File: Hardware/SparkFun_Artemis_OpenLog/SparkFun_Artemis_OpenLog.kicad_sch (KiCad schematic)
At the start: 100 parts, among them J1 CONN_021X02_NO_SILK, J11 QWIIC_CONNECTORJS-1MM, J14 CORTEX_JTAG, J2 JST_2MM_MALE, J3 CONN_021X02_NO_SILK, J4 CONN_06NO_SILK_NO_POP, J5 USB_C_4-LAYER_PADS, J6 MICRO-SD, J7 CONN_01PTH_NO_SILK_YES_STOP, Q1 20V/0.2A/8MHz/1.2Ω/1Vth, Q10 20V/0.2A/8MHz/1.2Ω/1Vth, Q2 20V/4.2A/52mΩ/1.4W, Q3 20V/0.2A/8MHz/1.2Ω/1Vth, Q7 20V/0.2A/8MHz/1.2Ω/1Vth, Q9 20V/0.2A/8MHz/1.2Ω/1Vth, U1 3.0V Supervisor, U10 CH340E, U13 9DoF IMU, U14 1.8V/100mA, U2 MCP73831, U3 3.3V, U4 3.3V, U8 ARTEMIS_MODULE, Y3 32.768kHz

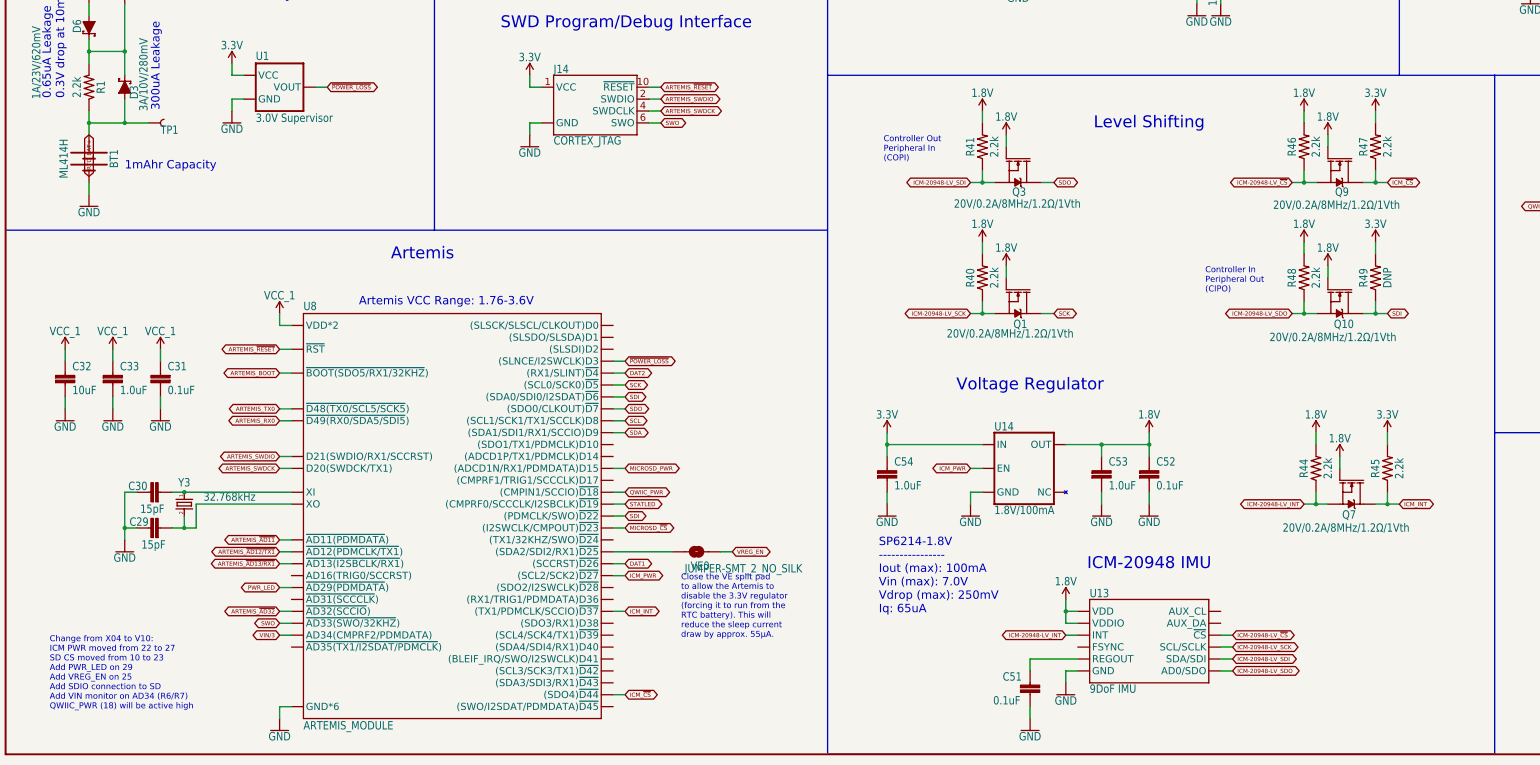
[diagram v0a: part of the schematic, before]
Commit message: Updates the design export
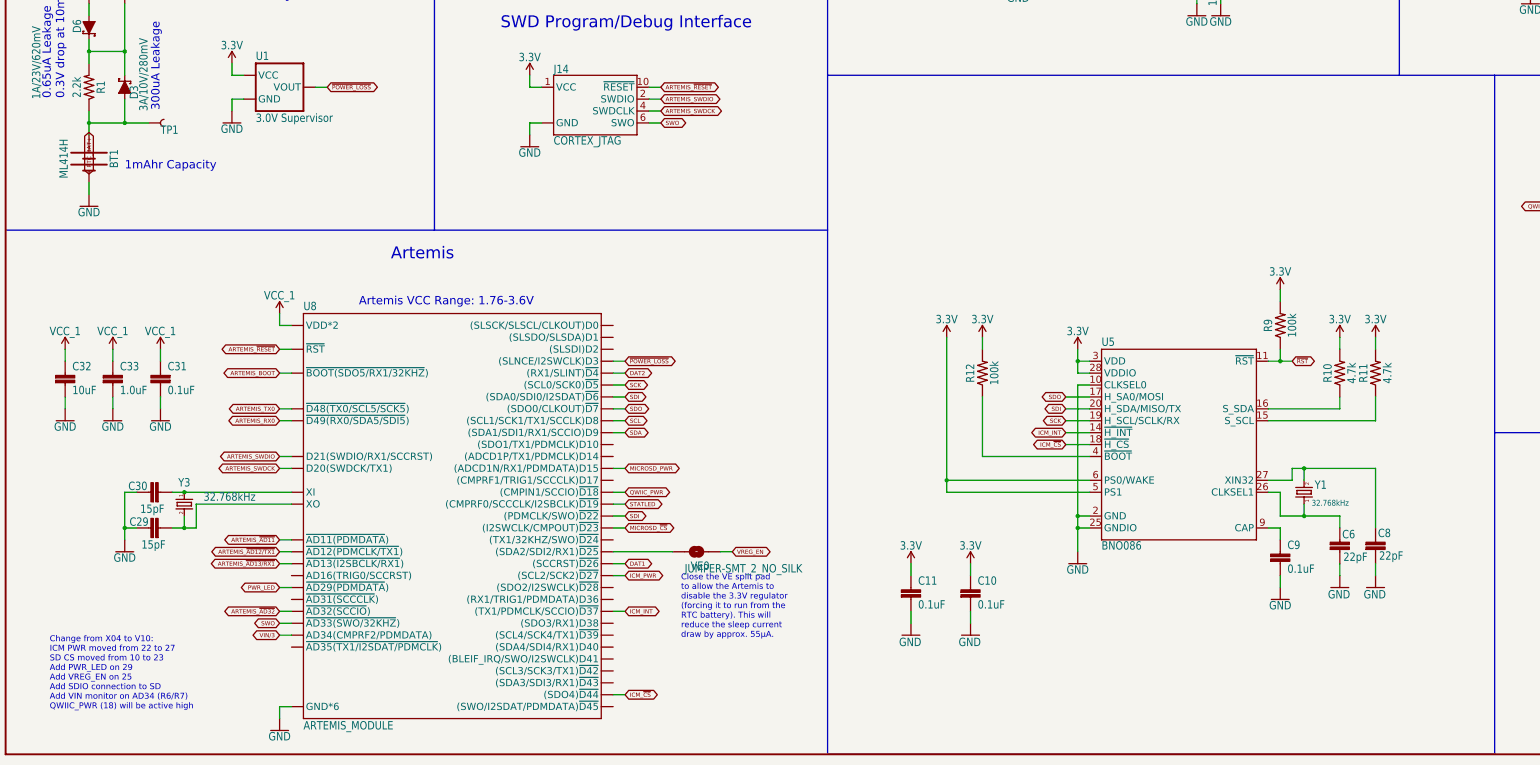
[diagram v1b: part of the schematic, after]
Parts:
- removed C51, C52: 0.1uF, SparkFun_Artemis_OpenLog:0402-TIGHT, symbol SparkFun_Artemis_OpenLog-eagle-import:0.1UF-0402T-16V-10%
- removed C53, C54: 1.0uF, SparkFun_Artemis_OpenLog:0402-TIGHT, symbol SparkFun_Artemis_OpenLog-eagle-import:1.0UF-0402T-16V-10%
- removed Q1, Q10, Q3, Q7, Q9: 20V/0.2A/8MHz/1.2Ω/1Vth, SparkFun_Artemis_OpenLog:SOT-416FL, symbol SparkFun_Artemis_OpenLog-eagle-import:MOSFET-NCH-RE1C00UNTL
- removed R40, R41, R44, R45, R46, R47, R48: 2.2k, SparkFun_Artemis_OpenLog:0402-TIGHT, symbol SparkFun_Artemis_OpenLog-eagle-import:2.2KOHM-0402T-1/16W-1%
- removed R49: DNP, SparkFun_Artemis_OpenLog:0402-TIGHT, symbol SparkFun_Artemis_OpenLog-eagle-import:RESISTOR0402T
- removed U13: 9DoF IMU, SparkFun_Artemis_OpenLog:QFN24-3X3-ICM-20948, symbol SparkFun_Artemis_OpenLog-eagle-import:ICM-20948
- removed U14: 1.8V/100mA, SparkFun_Artemis_OpenLog:SC70, symbol SparkFun_Artemis_OpenLog-eagle-import:V_REG_SP6214-1.8V
- added C10, C11, C9: 0.1uF, SparkFun_Artemis_OpenLog:0402, symbol SparkFun_Artemis_OpenLog-eagle-import:0.1UF-0402-6.3V-10%-X7R
- added C6, C8: 22pF, SparkFun_Artemis_OpenLog:0402-TIGHT, symbol SparkFun_Artemis_OpenLog-eagle-import:22PF-0402T-16V-10%
- added R10, R11: 4.7k, SparkFun_Artemis_OpenLog:0402-TIGHT, symbol SparkFun_Artemis_OpenLog-eagle-import:4.7KOHM-0402T-1/16W-1%
- added R12, R9: 100k, SparkFun_Artemis_OpenLog:0402-TIGHT, symbol SparkFun_Artemis_OpenLog-eagle-import:100KOHM-0402T-1/16W-1%
- added U5: BNO086, SparkFun_Artemis_OpenLog:LGA-28, symbol SparkFun_Artemis_OpenLog-eagle-import:BNO086
- added Y1: 32.768kHz, SparkFun_Artemis_OpenLog:CRYSTAL-SMD-3.2X1.5MM, symbol SparkFun_Artemis_OpenLog-eagle-import:CRYSTAL-32.768KHZSMD-3.2X1.5
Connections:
- net 3.3V: now also C10.1, C11.1, R10.2, R11.2, R12.2, R9.2, U5.28 (VDDIO), U5.3 (VDD), U5.5 (PS1), U5.6 (PS0/WAKE)
- net GND: now also C10.2, C11.2, C6.2, C8.2, C9.2, U5.10 (CLKSEL0), U5.2 (GND), U5.25 (GNDIO)
- net ICM_INT: now also U5.14 (~{H_INT})
- net ICM_~{CS}: now also U5.18 (~{H_CS})
- net SCK: now also U5.19 (H_SCL/SCLK/RX)
- net SDI: now also U5.20 (H_SDA/MISO/TX)
- net SDO: now also U5.17 (H_SA0/MOSI)
- new net: C6.1, U5.26 (CLKSEL1), Y1.P$1 (1)
- new net: C8.1, U5.27 (XIN32), Y1.P$2 (2)
- new net: R11.1, U5.15 (S_SCL)
- new net: R10.1, U5.16 (S_SDA)
- new net: R12.1, U5.4 (~{BOOT})
- new net: C9.1, U5.9 (CAP)
- new net ~{RST}: R9.1, U5.11 (~{RST})
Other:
- note removed: "Controller In Peripheral Out (CIPO)"
- note removed: "Controller Out Peripheral In (COPI)"
- note removed: "ICM-20948 IMU"
- note removed: "Level Shifting"
- note removed: "SP6214-1.8V ---------------- Iout (max): 100mA Vin (max): 7.0V Vdrop (max): 250mV Iq: 65uA"
- note removed: "Voltage Regulator"

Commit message: Generates footprint library, updates many parts from the SparkFun KiCaad libraries
* This is just a save point
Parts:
- removed unit 1 of FRAME1
- removed J1: CONN_021X02_NO_SILK, SparkFun_Artemis_OpenLog:1X02_NO_SILK, symbol SparkFun_Artemis_OpenLog-eagle-import:CONN_021X02_NO_SILK
- removed J2: JST_2MM_MALE, SparkFun_Artemis_OpenLog:JST-2-SMD, symbol SparkFun_Artemis_OpenLog-eagle-import:JST_2MM_MALE
- removed J5: USB_C_4-LAYER_PADS, SparkFun_Artemis_OpenLog:USB-C-16P_4LAYER-PADS, symbol SparkFun_Artemis_OpenLog-eagle-import:USB_C_4-LAYER_PADS
- added J2: Conn_01x02, SparkFun-Connector:1x02_P2.54mm, symbol SparkFun-Connector:Conn_01x02_P2.54mm
- added J5: JST_2mm_LiPo, SparkFun-Connector:JST_1x02_P2.0mm_Horizontal_SMD, symbol SparkFun-Connector:Conn_01x02_JST_P2.0mm_Horizontal_SMD_LiPo
- added J8: USB_C_Receptacle, SparkFun-Connector:USB-C_16, symbol SparkFun-Connector:USB_C_Receptacle
- BT1: footprint SparkFun_Artemis_OpenLog:ML414H_IV01E -> SparkFun-Battery:ML414H_IV01E; symbol SparkFun_Artemis_OpenLog-eagle-import:ML414H_IV01E_BATTERY -> SparkFun-Battery:Battery_6.8mm_ML414H_IV01E
- C31, C41, C42, C43, C46: footprint SparkFun_Artemis_OpenLog:0402-TIGHT -> SparkFun-Capacitor:C_0402_1005Metric; symbol SparkFun_Artemis_OpenLog-eagle-import:0.1UF-0402T-16V-10% -> SparkFun-Capacitor:0.1uF_0402_16V_10%; PROD_ID CAP-12416 -> CAP-25565; Tolerance (none) -> 10%; Voltage (none) -> 16V
- C44: footprint SparkFun_Artemis_OpenLog:0402-TIGHT -> SparkFun-Capacitor:C_0402_1005Metric; symbol SparkFun_Artemis_OpenLog-eagle-import:1.0NF/1000PF-0402_TIGHT-50V-10% -> SparkFun-Capacitor:1.0nF_0402_50V_10%; Tolerance (none) -> 10%; Voltage (none) -> 50V
- J11: value QWIIC_CONNECTORJS-1MM -> Qwiic_RA; footprint SparkFun_Artemis_OpenLog:JST04_1MM_RA -> SparkFun-Connector:JST_1x04_P1.0mm_Horizontal_SMD; symbol SparkFun_Artemis_OpenLog-eagle-import:QWIIC_CONNECTORJS-1MM -> SparkFun-Connector:Qwiic_Horizontal
- J3: value CONN_021X02_NO_SILK -> Conn_01x02; footprint SparkFun_Artemis_OpenLog:1X02_NO_SILK -> SparkFun-Connector:1x02_P2.54mm; symbol SparkFun_Artemis_OpenLog-eagle-import:CONN_021X02_NO_SILK -> SparkFun-Connector:Conn_01x02_P2.54mm
- R22, R23, R24, R25, R5: footprint SparkFun_Artemis_OpenLog:0402-TIGHT -> SparkFun-Resistor:R_0402_1005Metric; symbol SparkFun_Artemis_OpenLog-eagle-import:1KOHM-0402T-1/16W-1% -> SparkFun-Resistor:1k_0402
- R26, R27: footprint SparkFun_Artemis_OpenLog:0402-TIGHT -> SparkFun-Resistor:R_0402_1005Metric; symbol SparkFun_Artemis_OpenLog-eagle-import:5.1KOHM-0402T-1/16W-1% -> SparkFun-Resistor:5.1k_0402
- U2: footprint SparkFun_Artemis_OpenLog:SOT23-5 -> SparkFun-Semiconductor-Standard:SOT23-5; symbol SparkFun_Artemis_OpenLog-eagle-import:MCP73831 -> SparkFun-IC-Power:MCP73831
- U3: value 3.3V -> AP2112K-3.3; footprint SparkFun_Artemis_OpenLog:SOT23-5 -> SparkFun-Semiconductor-Standard:SOT23-5; symbol SparkFun_Artemis_OpenLog-eagle-import:V_REG_AP2112K-3.3V -> SparkFun-Regulator:AP2112K-3.3; IMax (none) -> 600mA; Iq (none) -> 55µA; VMax (none) -> 6V
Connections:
- net 5V: now also J8.VBUS
- net GND: now also J2.2 (Pin_2), J5.2 (+), J8.GND
- net V_BATT: now also J2.1 (Pin_1), J5.1 (-)
- net at R27.2: now also J8.A5 (CC1)
- net at R26.2: now also J8.B5 (CC2)
- net at R8.2: now also J8.S (SHIELD)
- net at U10.1 (UD+): now also J8.A6 (D+), J8.B6 (D+)
- net at U10.2 (UD-): now also J8.A7 (D-), J8.B7 (D-)
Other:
- moved on the sheet: D1, R4, R8

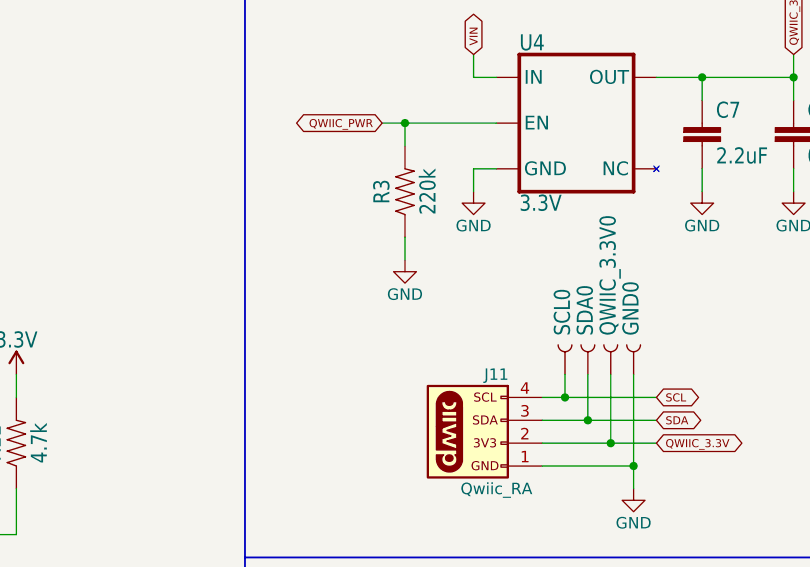
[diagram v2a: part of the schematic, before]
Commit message: Another save point
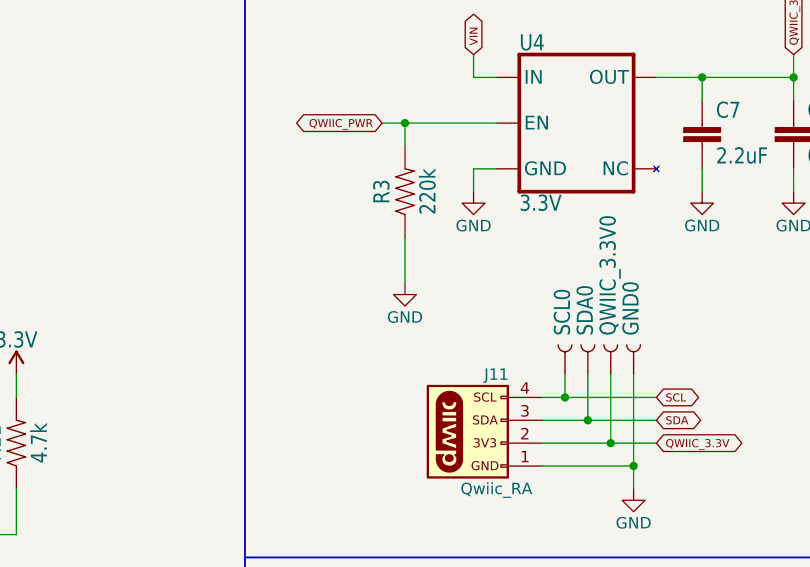
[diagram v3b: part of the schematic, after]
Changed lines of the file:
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@@
 	(wire
 		(pts
+			(xy 353.06 193.04) (xy 353.06 198.12)
+		)
+		(stroke
+			(width 0.1524)
+			(type solid)
+		)
+	)
+	(wire
+		(pts
 			(xy 294.64 236.22) (xy 292.1 236.22)
 		)
@@
 	(wire
 		(pts
-			(xy 353.06 195.58) (xy 353.06 193.04)
-		)
-		(stroke
-			(width 0.1524)
-			(type solid)
-		)
-	)
-	(wire
-		(pts
 			(xy 353.06 43.18) (xy 350.52 43.18)
 		)
@@
 	(symbol
 		(lib_id "SparkFun-PowerSymbol:GND")
-		(at 353.06 195.58 0)
+		(at 353.06 198.12 0)
 		(unit 1)
 		(body_style 1)
@@
 		(dnp no)
 		(property "Reference" "#PWR9"
-			(at 353.06 201.93 0)
+			(at 353.06 204.47 0)
 			(hide yes)
 			(show_name no)
@@
 		)
 		(property "Value" "GND"
-			(at 353.06 199.39 0)
+			(at 353.06 201.93 0)
 			(show_name no)
 			(do_not_autoplace yes)
@@
 		)
 		(property "Footprint" ""
-			(at 353.06 195.58 0)
+			(at 353.06 198.12 0)
 			(hide yes)
 			(show_name no)
@@
 		)
 		(property "Datasheet" ""
-			(at 353.06 195.58 0)
+			(at 353.06 198.12 0)
 			(hide yes)
 			(show_name no)
@@
 		)
 		(property "Description" "Power symbol creates a global label with name \"GND\" , ground"
-			(at 353.06 204.47 0)
+			(at 353.06 207.01 0)
 			(hide yes)
 			(show_name no)
